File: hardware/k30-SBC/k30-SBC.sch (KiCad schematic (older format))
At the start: 17 parts, among them SW1 RESET, U1 MC68030FE, U2 74HC14, U3 74HC05, Y1 Crystal

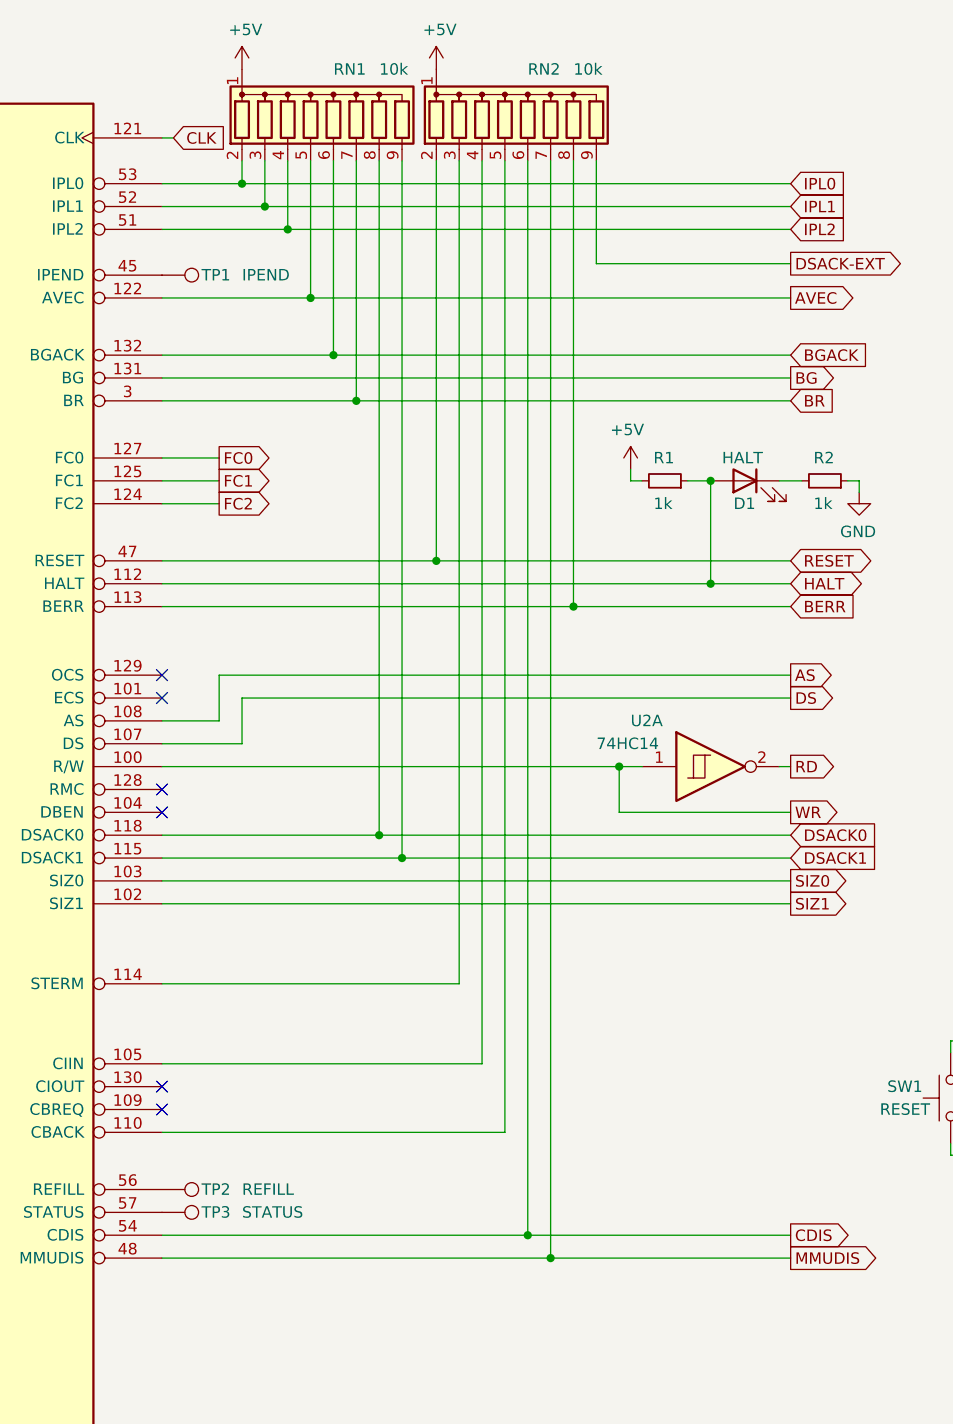
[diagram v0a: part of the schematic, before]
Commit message: Almost completed k30-SBC board design
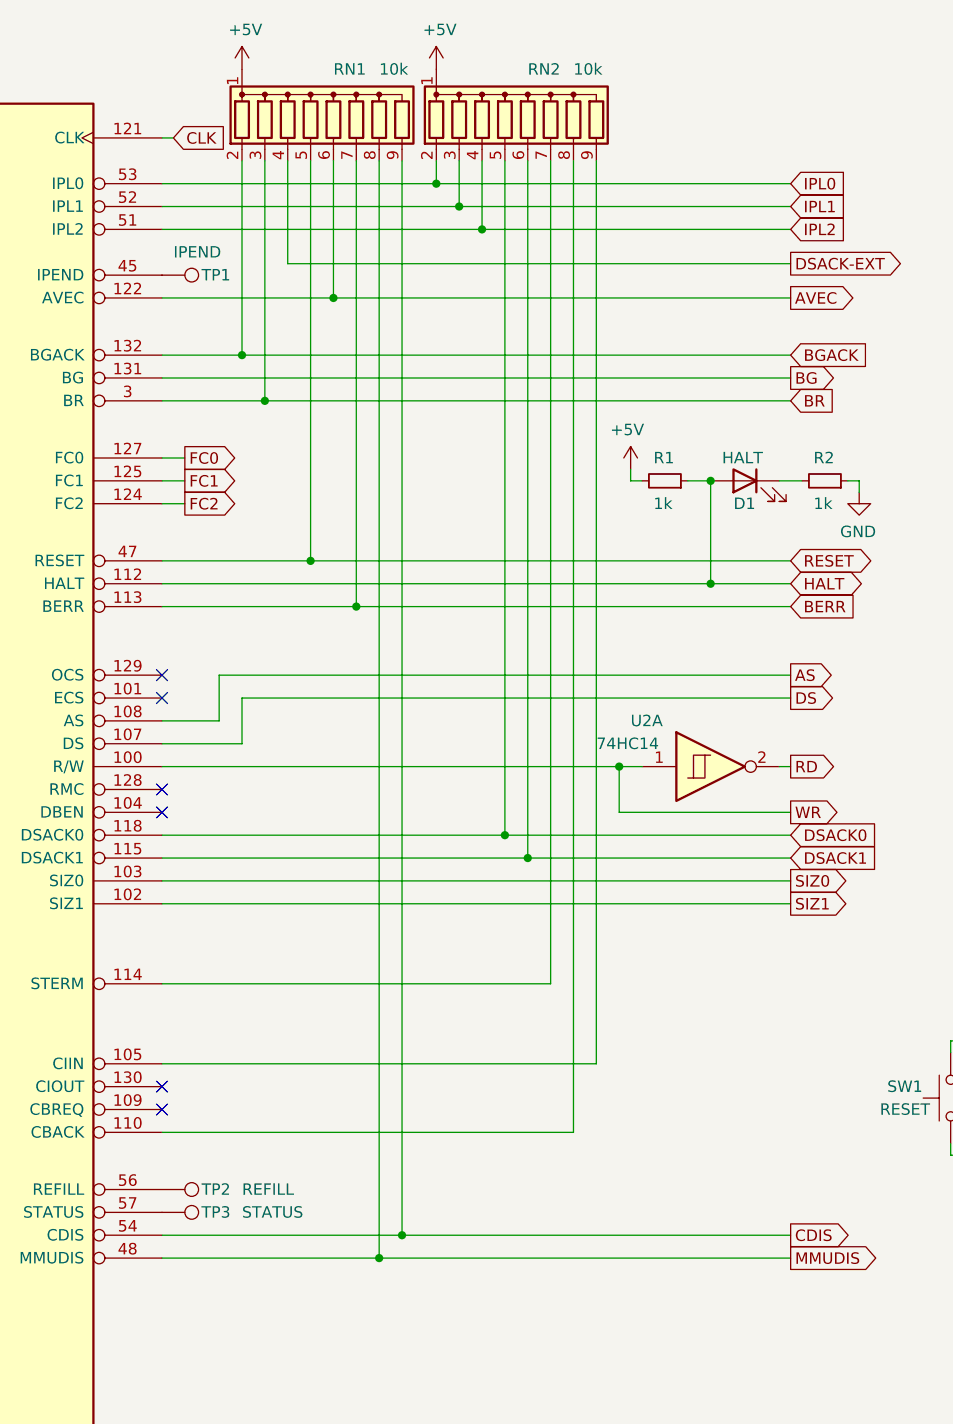
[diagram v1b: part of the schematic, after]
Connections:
- net AVEC: now also RN1.6 (R5); no longer RN1.5 (R4)
- net BERR: now also RN1.7 (R6); no longer RN2.8 (R7)
- net BGACK: now also RN1.2 (R1); no longer RN1.6 (R5)
- net BR: now also RN1.3 (R2); no longer RN1.7 (R6)
- net CDIS: now also RN1.9 (R8); no longer RN2.6 (R5)
- net DSACK-EXT: now also RN1.4 (R3); no longer RN2.9 (R8)
- net DSACK0: now also RN2.5 (R4); no longer RN1.8 (R7)
- net DSACK1: now also RN2.6 (R5); no longer RN1.9 (R8)
- net IPL0: now also RN2.2 (R1); no longer RN1.2 (R1)
- net IPL1: now also RN2.3 (R2); no longer RN1.3 (R2)
- net IPL2: now also RN2.4 (R3); no longer RN1.4 (R3)
- net MMUDIS: now also RN1.8 (R7); no longer RN2.7 (R6)
- net RESET: now also RN1.5 (R4); no longer RN2.2 (R1)
- net at U1.105 (CIIN): now also RN2.9 (R8); no longer RN2.4 (R3)
- net at U1.110 (CBACK): now also RN2.8 (R7); no longer RN2.5 (R4)
- net at U1.114 (STERM): now also RN2.7 (R6); no longer RN2.3 (R2)
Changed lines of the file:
@@
 	7900 2500 7800 2500
 Wire Wire Line
-	6300 1100 6300 2850
+	5750 1100 5750 2850
 Wire Wire Line
 	5450 3450 7850 3450
@@
 DSACK1
 Wire Wire Line
-	6400 1100 6400 4700
-Wire Wire Line
-	6400 4700 5100 4700
-Wire Wire Line
-	5100 5050 6500 5050
-Wire Wire Line
-	6500 5050 6500 1100
-Wire Wire Line
-	5100 5350 6600 5350
-Wire Wire Line
-	6600 5350 6600 1100
-Wire Wire Line
-	6700 5800 6700 1100
-Wire Wire Line
-	6800 5900 6800 1100
-$Comp
-L Device:R_Network08 RN2
-U 1 1 615B22B4
-P 6700 900
-F 0 "RN2" H 6700 1100 50  0000 L CNN
-F 1 "10k" H 6900 1100 50  0000 L CNN
-F 2 "Resistor_THT:R_Array_SIP9" V 7175 900 50  0001 C CNN
-F 3 "http://www.vishay.com/docs/31509/csc.pdf" H 6700 900 50  0001 C CNN
-	1    6700 900
-	1    0    0    -1
-$EndComp
-Wire Wire Line
-	6150 1100 6150 4150
-Wire Wire Line
-	5100 2850 6300 2850
-Wire Wire Line
-	5100 4150 6150 4150
+	6800 1100 6800 4700
+Wire Wire Line
+	6800 4700 5100 4700
+Wire Wire Line
+	6700 1100 6700 4150
 $Comp
 L power:+5V #PWR03
@@
 	1    0    0    -1
 $EndComp
-$Comp
-L Device:R_Network08 RN1
-U 1 1 61F69B4D
-P 5850 900
-F 0 "RN1" H 5850 1100 50  0000 L CNN
-F 1 "10k" H 6050 1100 50  0000 L CNN
-F 2 "Resistor_THT:R_Array_SIP9" V 6325 900 50  0001 C CNN
-F 3 "http://www.vishay.com/docs/31509/csc.pdf" H 5850 900 50  0001 C CNN
-	1    5850 900
-	1    0    0    -1
-$EndComp
-Connection ~ 6300 2850
-Wire Wire Line
-	5100 1200 5450 1200
-Wire Wire Line
-	5450 1200 5450 1100
-Wire Wire Line
-	5100 1300 5550 1300
-Wire Wire Line
-	5550 1300 5550 1100
-Wire Wire Line
-	5100 1400 5650 1400
-Wire Wire Line
-	5650 1400 5650 1100
-Wire Wire Line
-	5450 1200 7850 1200
-Connection ~ 5450 1200
 Text GLabel 7850 1200 2    50   Input ~ 0
 IPL0
@@
 Text GLabel 7850 1400 2    50   Input ~ 0
 IPL2
-Wire Wire Line
-	5550 1300 7850 1300
-Connection ~ 5550 1300
-Wire Wire Line
-	5650 1400 7850 1400
-Connection ~ 5650 1400
 Text GLabel 7850 1950 2    50   Input ~ 0
 BGACK
@@
 	5100 2050 7850 2050
 Wire Wire Line
-	5850 1950 5850 1100
-Wire Wire Line
-	5950 2150 5950 1100
+	5450 1950 5450 1100
+Wire Wire Line
+	5550 2150 5550 1100
 Wire Wire Line
 	7150 2500 7200 2500
@@
 	7400 2500 7500 2500
 Wire Wire Line
-	5100 2400 5350 2400
-Text GLabel 5350 2400 2    50   Output ~ 0
+	5100 2400 5200 2400
+Text GLabel 5200 2400 2    50   Output ~ 0
 FC0
-Text GLabel 5350 2500 2    50   Output ~ 0
+Text GLabel 5200 2500 2    50   Output ~ 0
 FC1
-Text GLabel 5350 2600 2    50   Output ~ 0
+Text GLabel 5200 2600 2    50   Output ~ 0
 FC2
 Wire Wire Line
-	5100 2500 5350 2500
-Wire Wire Line
-	5100 2600 5350 2600
+	5100 2500 5200 2500
+Wire Wire Line
+	5100 2600 5200 2600
 Text GLabel 7850 3050 2    50   Input ~ 0
 BERR
@@
 NoConn ~ 5100 3850
 NoConn ~ 5100 3950
-Wire Wire Line
-	5100 1700 5750 1700
-Wire Wire Line
-	5750 1700 5750 1100
 NoConn ~ 5100 5150
 NoConn ~ 5100 5250
-Wire Wire Line
-	5100 1950 5850 1950
-Wire Wire Line
-	5100 2150 5950 2150
-Connection ~ 5850 1950
-Connection ~ 5950 2150
-Wire Wire Line
-	5850 1950 7850 1950
-Wire Wire Line
-	5950 2150 7850 2150
-$Comp
-L Connector:TestPoint TP?
-U 1 1 61A7716E
-P 5100 1600
-AR Path="/613AFF13/61A7716E" Ref="TP?"  Part="1"
-AR Path="/61A7716E" Ref="TP1"  Part="1"
-F 0 "TP1" V 5100 1900 50  0000 R CNN
-F 1 "IPEND" V 5100 1950 50  0000 L CNN
-F 2 "TestPoint:TestPoint_THTPad_2.0x2.0mm_Drill1.0mm" H 5300 1600 50  0001 C CNN
-F 3 "~" H 5300 1600 50  0001 C CNN
-	1    5100 1600
-	0    1    1    0
-$EndComp
 Text GLabel 7850 1550 2    50   Output ~ 0
 DSACK-EXT
@@
 	5450 3650 5450 3450
 Wire Wire Line
-	6300 2850 7850 2850
-Wire Wire Line
-	5100 4050 6050 4050
-Wire Wire Line
-	6050 1100 6050 4050
-Connection ~ 6050 4050
-Connection ~ 6150 4150
-Wire Wire Line
-	6150 4150 7850 4150
-Wire Wire Line
-	6050 4050 7850 4050
+	6600 1100 6600 4050
 Text GLabel 7850 1700 2    50   Output ~ 0
 AVEC
-Wire Wire Line
-	5750 1700 7850 1700
-Connection ~ 5750 1700
-Wire Wire Line
-	7000 1100 7000 1550
-Wire Wire Line
-	7000 1550 7850 1550
 Wire Wire Line
 	5350 3350 5350 3550
@@
 	1    0    0    -1
 $EndComp
-Wire Wire Line
-	5100 3050 6900 3050
-Wire Wire Line
-	6900 1100 6900 3050
-Connection ~ 6900 3050
-Wire Wire Line
-	6900 3050 7850 3050
 Text GLabel 7850 5900 2    50   Output ~ 0
 MMUDIS
 Text GLabel 7850 5800 2    50   Output ~ 0
 CDIS
-Wire Wire Line
-	6700 5800 7850 5800
-Connection ~ 6700 5800
-Wire Wire Line
-	6800 5900 7850 5900
-Connection ~ 6800 5900
-Wire Wire Line
-	5100 5900 6800 5900
-Wire Wire Line
-	5100 5800 6700 5800
+$Comp
+L Connector:TestPoint TP?
+U 1 1 61A7716E
+P 5100 1600
+AR Path="/613AFF13/61A7716E" Ref="TP?"  Part="1"
+AR Path="/61A7716E" Ref="TP1"  Part="1"
+F 0 "TP1" V 5100 1900 50  0000 R CNN
+F 1 "IPEND" V 5000 1650 50  0000 L CNN
+F 2 "TestPoint:TestPoint_THTPad_2.0x2.0mm_Drill1.0mm" H 5300 1600 50  0001 C CNN
+F 3 "~" H 5300 1600 50  0001 C CNN
+	1    5100 1600
+	0    1    1    0
+$EndComp
+Wire Wire Line
+	6500 1400 6500 1100
+Wire Wire Line
+	6400 1300 6400 1100
+Wire Wire Line
+	6300 1200 6300 1100
+$Comp
+L Device:R_Network08 RN2
+U 1 1 615B22B4
+P 6700 900
+F 0 "RN2" H 6700 1100 50  0000 L CNN
+F 1 "10k" H 6900 1100 50  0000 L CNN
+F 2 "Resistor_THT:R_Array_SIP9" V 7175 900 50  0001 C CNN
+F 3 "http://www.vishay.com/docs/31509/csc.pdf" H 6700 900 50  0001 C CNN
+	1    6700 900
+	1    0    0    -1
+$EndComp
+Wire Wire Line
+	7000 1100 7000 5050
+Wire Wire Line
+	5100 5050 7000 5050
+Wire Wire Line
+	6900 5350 6900 1100
+Wire Wire Line
+	5100 5350 6900 5350
+Connection ~ 6600 4050
+Wire Wire Line
+	6600 4050 7850 4050
+Connection ~ 6700 4150
+Wire Wire Line
+	6700 4150 7850 4150
+Wire Wire Line
+	5100 4150 6700 4150
+Wire Wire Line
+	5100 4050 6600 4050
+Wire Wire Line
+	6050 1100 6050 5900
+Wire Wire Line
+	5100 5900 6050 5900
+Wire Wire Line
+	5100 3050 5950 3050
+Wire Wire Line
+	5850 1100 5850 1700
+Wire Wire Line
+	5950 3050 5950 1100
+Connection ~ 5950 3050
+Wire Wire Line
+	5950 3050 7850 3050
+Connection ~ 6050 5900
+Wire Wire Line
+	6050 5900 7850 5900
+Wire Wire Line
+	6150 1100 6150 5800
+Wire Wire Line
+	5100 5800 6150 5800
+Connection ~ 6150 5800
+Wire Wire Line
+	6150 5800 7850 5800
+Wire Wire Line
+	5100 1400 6500 1400
+Wire Wire Line
+	5100 1300 6400 1300
+Wire Wire Line
+	5100 1200 6300 1200
+$Comp
+L Device:R_Network08 RN1
+U 1 1 61F69B4D
+P 5850 900
+F 0 "RN1" H 5850 1100 50  0000 L CNN
+F 1 "10k" H 6050 1100 50  0000 L CNN
+F 2 "Resistor_THT:R_Array_SIP9" V 6325 900 50  0001 C CNN
+F 3 "http://www.vishay.com/docs/31509/csc.pdf" H 5850 900 50  0001 C CNN
+	1    5850 900
+	1    0    0    -1
+$EndComp
+Wire Wire Line
+	5650 1100 5650 1550
+Connection ~ 6300 1200
+Wire Wire Line
+	6300 1200 7850 1200
+Connection ~ 6400 1300
+Wire Wire Line
+	6400 1300 7850 1300
+Connection ~ 6500 1400
+Wire Wire Line
+	6500 1400 7850 1400
+Wire Wire Line
+	5100 1950 5450 1950
+Wire Wire Line
+	5100 2150 5550 2150
+Wire Wire Line
+	5650 1550 7850 1550
+Connection ~ 5750 2850
+Wire Wire Line
+	5750 2850 7850 2850
+Connection ~ 5850 1700
+Wire Wire Line
+	5850 1700 7850 1700
+Wire Wire Line
+	5100 1700 5850 1700
+Wire Wire Line
+	5100 2850 5750 2850
+Connection ~ 5450 1950
+Wire Wire Line
+	5450 1950 7850 1950
+Connection ~ 5550 2150
+Wire Wire Line
+	5550 2150 7850 2150
 Wire Bus Line
 	1600 900  1600 7200
